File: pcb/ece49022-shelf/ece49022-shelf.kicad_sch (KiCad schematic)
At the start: 15 parts

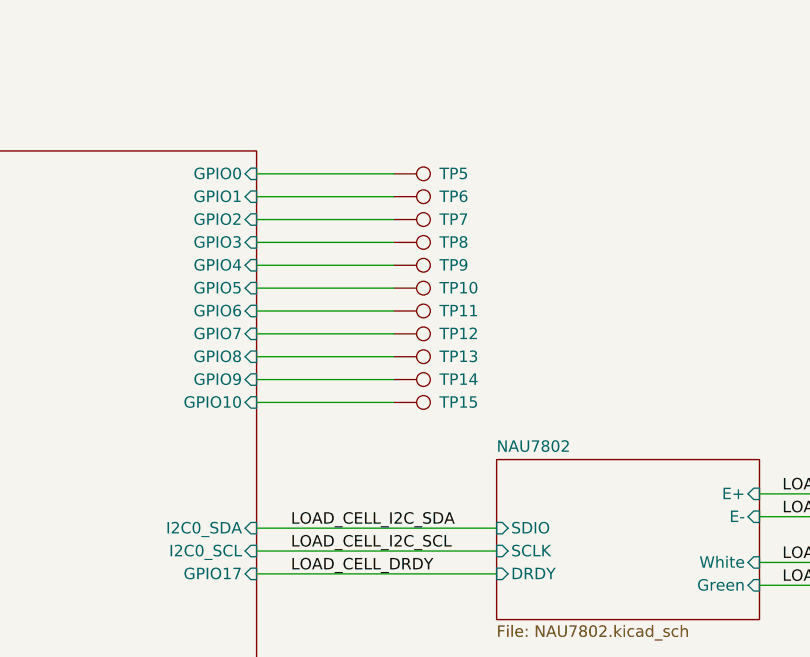
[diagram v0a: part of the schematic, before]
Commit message: added power
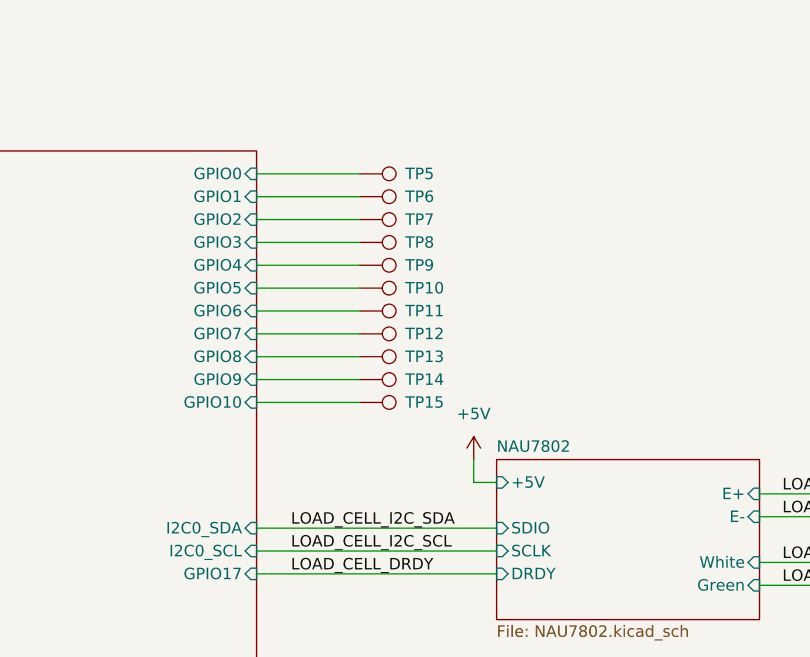
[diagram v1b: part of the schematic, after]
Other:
- sheet NAU7802 ports: added +5V; removed none
- moved on the sheet: TP10, TP11, TP12, TP13, TP14, TP15, TP5, TP6, TP7, TP8, TP9

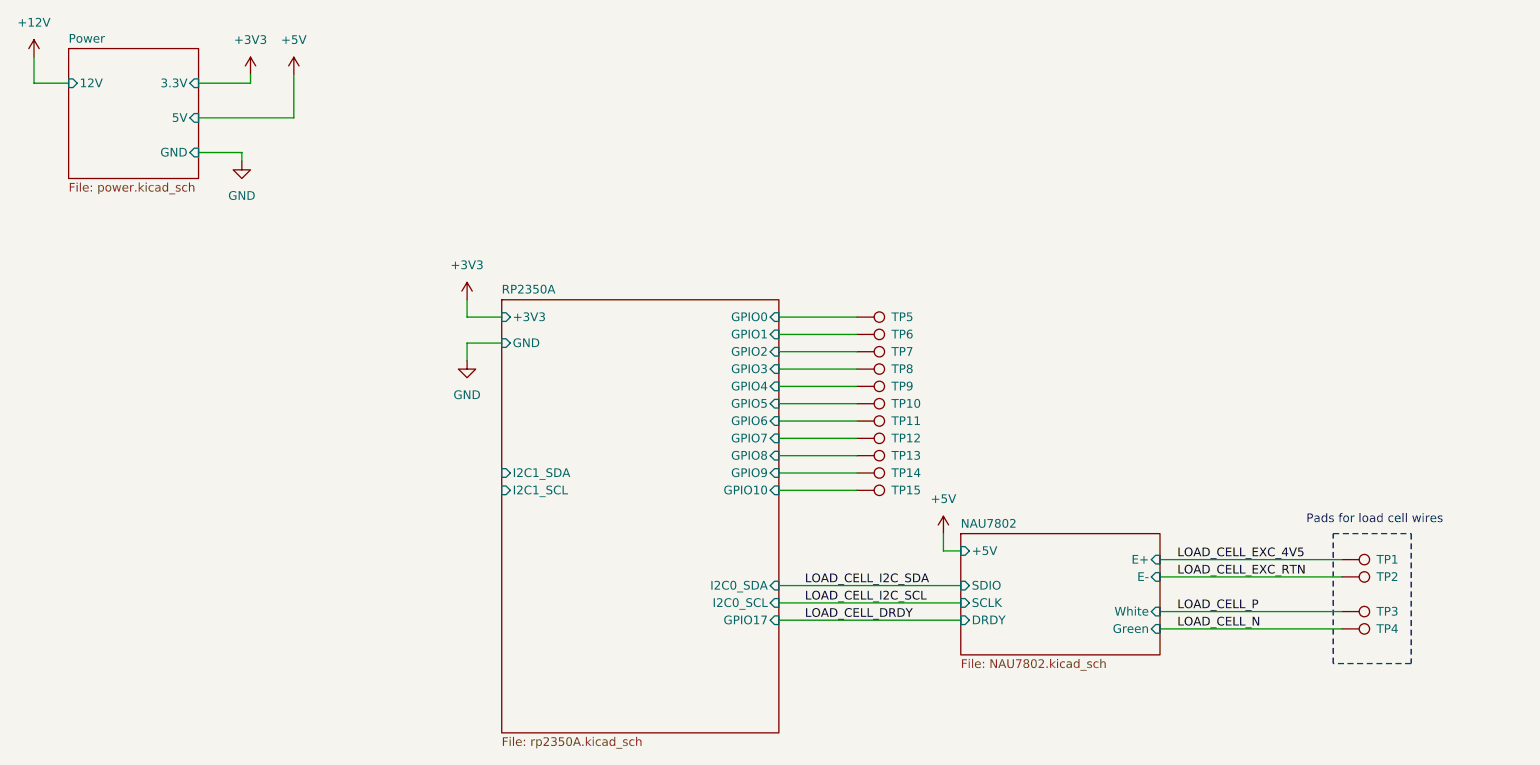
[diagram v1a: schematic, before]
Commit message: test
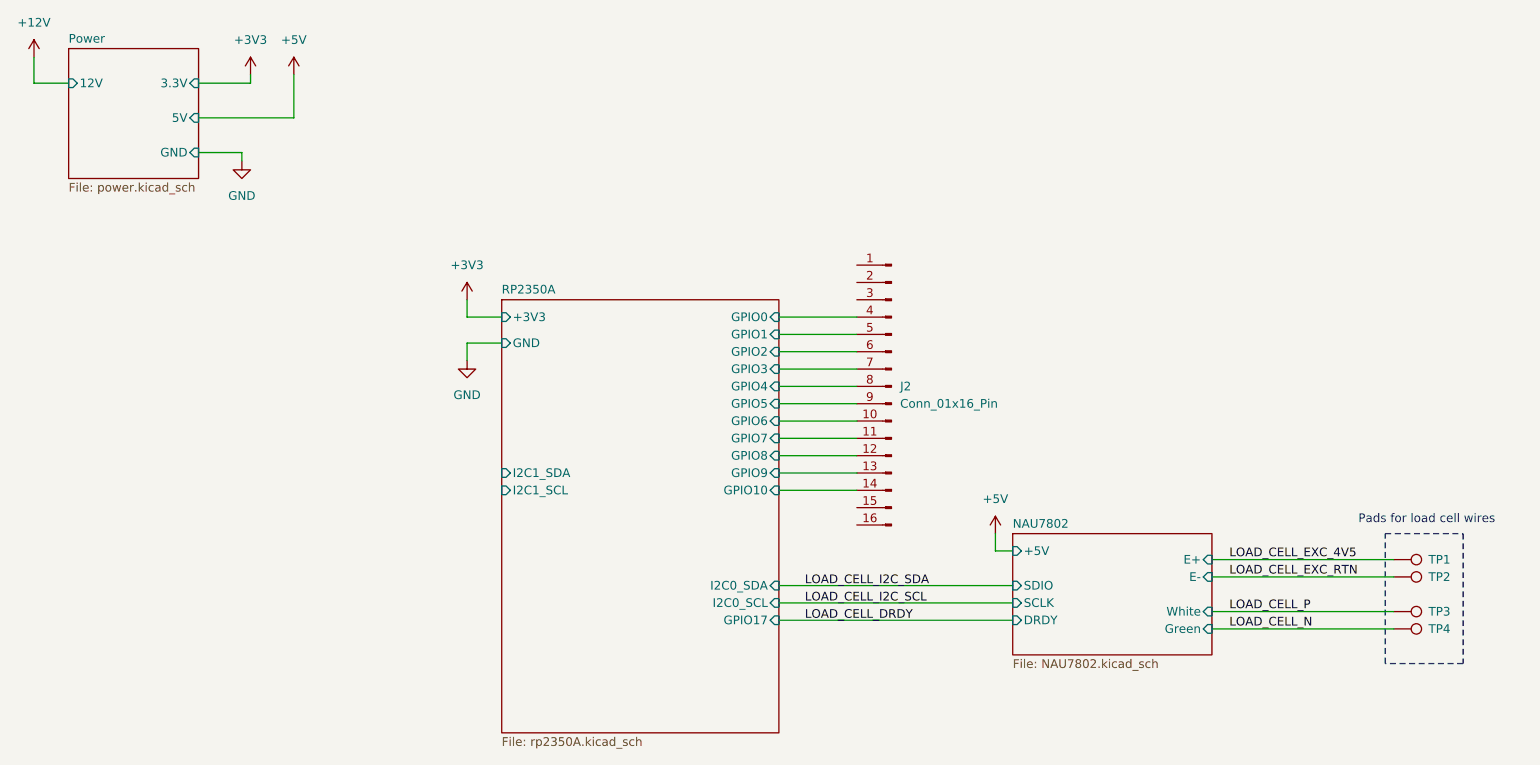
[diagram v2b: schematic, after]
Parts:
- removed TP10, TP11, TP12, TP13, TP14, TP15, TP5, TP6, TP7, TP8, TP9: TestPoint, symbol Connector:TestPoint
- added J2: Conn_01x16_Pin, symbol Connector:Conn_01x16_Pin
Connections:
- net RP2350A/GPIO0: now also J2.4 (Pin_4)
- net RP2350A/GPIO1: now also J2.5 (Pin_5)
- net RP2350A/GPIO10: now also J2.14 (Pin_14)
- net RP2350A/GPIO2: now also J2.6 (Pin_6)
- net RP2350A/GPIO3: now also J2.7 (Pin_7)
- net RP2350A/GPIO4: now also J2.8 (Pin_8)
- net RP2350A/GPIO5: now also J2.9 (Pin_9)
- net RP2350A/GPIO6: now also J2.10 (Pin_10)
- net RP2350A/GPIO7: now also J2.11 (Pin_11)
- net RP2350A/GPIO8: now also J2.12 (Pin_12)
- net RP2350A/GPIO9: now also J2.13 (Pin_13)
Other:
- moved on the sheet: TP1, TP2, TP3, TP4
